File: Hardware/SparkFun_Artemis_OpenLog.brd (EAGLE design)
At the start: 30.5 x 30.5 mm, 126 parts, among them J14 CORTEX_JTAG, J6 MICRO-SD, Q1 20V/0.2A/8MHz/1.2Ω/1Vth, Q10 20V/0.2A/8MHz/1.2Ω/1Vth, Q2 20V/4.2A/52mΩ/1.4W, Q3 20V/0.2A/8MHz/1.2Ω/1Vth, Q7 20V/0.2A/8MHz/1.2Ω/1Vth, Q9 20V/0.2A/8MHz/1.2Ω/1Vth, U1 3.0V Supervisor, U10 CH340E, U13 ICM-20948, U14 1.8V/100mA, U2 MCP73831, U3 AP2112K, U4 AP2112K, U8 ARTEMIS_MODULE, Y3 32.768kHz

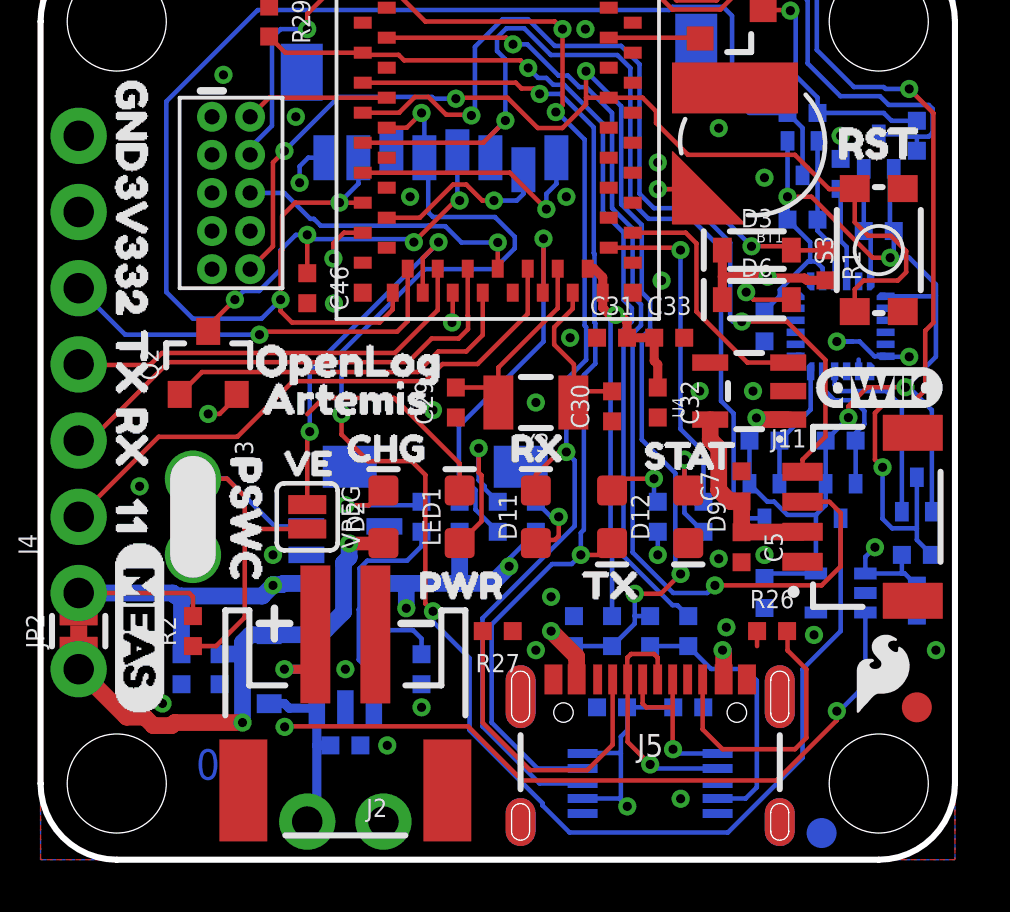
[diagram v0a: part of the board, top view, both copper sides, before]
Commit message: Update SparkFun_Artemis_OpenLog.brd
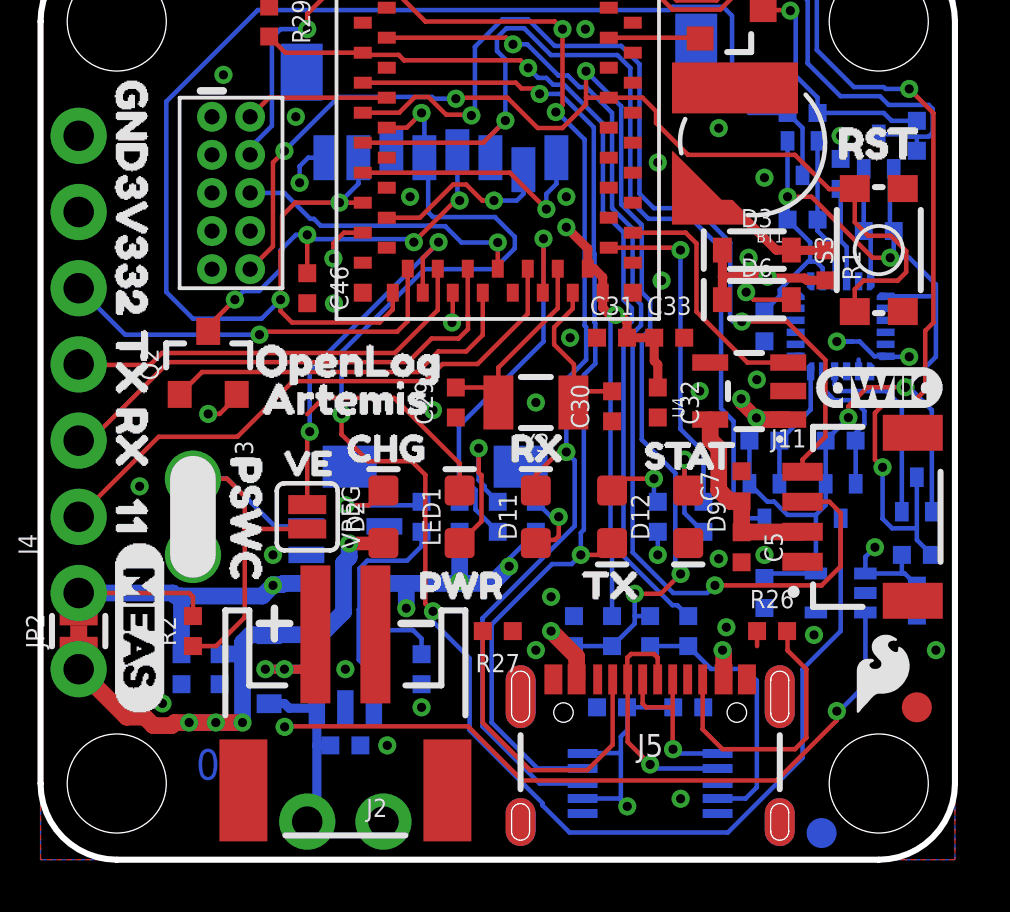
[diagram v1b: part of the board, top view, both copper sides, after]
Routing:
- net VCC_1: track 26.9 -> 33.2 mm, vias 2 -> 4
- net N$1: track 7.88 -> 5.07 mm, vias 2 -> 0
- net 5V: track 20.7 -> 22.5 mm, vias 4 -> 6
- net V_BATT: track 10.3 -> 11.6 mm, vias 1 -> 2
- net VIN: track 16.1 -> 17.0 mm, vias 2 -> 3
- net 3.3V: vias 8 -> 9
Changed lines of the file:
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@@
 <layers>
 <layer number="1" name="Top" color="4" fill="1" visible="yes" active="yes"/>
-<layer number="2" name="Vertical" color="1" fill="3" visible="no" active="yes"/>
-<layer number="15" name="Horz" color="4" fill="6" visible="no" active="yes"/>
+<layer number="2" name="Vertical" color="1" fill="3" visible="yes" active="yes"/>
+<layer number="15" name="Horz" color="4" fill="6" visible="yes" active="yes"/>
 <layer number="16" name="Bottom" color="1" fill="1" visible="yes" active="yes"/>
 <layer number="17" name="Pads" color="2" fill="1" visible="yes" active="yes"/>
@@
 <layer number="19" name="Unrouted" color="6" fill="1" visible="yes" active="yes"/>
 <layer number="20" name="Dimension" color="24" fill="1" visible="yes" active="yes"/>
-<layer number="21" name="tPlace" color="16" fill="1" visible="yes" active="yes"/>
-<layer number="22" name="bPlace" color="14" fill="1" visible="yes" active="yes"/>
-<layer number="23" name="tOrigins" color="15" fill="1" visible="yes" active="yes"/>
-<layer number="24" name="bOrigins" color="15" fill="1" visible="yes" active="yes"/>
+<layer number="21" name="tPlace" color="16" fill="1" visible="no" active="yes"/>
+<layer number="22" name="bPlace" color="14" fill="1" visible="no" active="yes"/>
+<layer number="23" name="tOrigins" color="15" fill="1" visible="no" active="yes"/>
+<layer number="24" name="bOrigins" color="15" fill="1" visible="no" active="yes"/>
 <layer number="25" name="tNames" color="7" fill="1" visible="no" active="yes"/>
 <layer number="26" name="bNames" color="7" fill="1" visible="no" active="yes"/>
@@
 <layer number="43" name="vRestrict" color="2" fill="10" visible="no" active="yes"/>
 <layer number="44" name="Drills" color="7" fill="1" visible="no" active="yes"/>
-<layer number="45" name="Holes" color="7" fill="1" visible="yes" active="yes"/>
+<layer number="45" name="Holes" color="7" fill="1" visible="no" active="yes"/>
 <layer number="46" name="Milling" color="3" fill="1" visible="no" active="yes"/>
 <layer number="47" name="Measures" color="7" fill="1" visible="no" active="yes"/>
 <layer number="48" name="Document" color="7" fill="1" visible="no" active="yes"/>
-<layer number="49" name="Reference" color="7" fill="1" visible="yes" active="yes"/>
+<layer number="49" name="Reference" color="7" fill="1" visible="no" active="yes"/>
 <layer number="50" name="dxf" color="7" fill="1" visible="no" active="yes"/>
-<layer number="51" name="tDocu" color="6" fill="1" visible="yes" active="yes"/>
+<layer number="51" name="tDocu" color="6" fill="1" visible="no" active="yes"/>
 <layer number="52" name="bDocu" color="7" fill="1" visible="no" active="yes"/>
 <layer number="91" name="Nets" color="2" fill="1" visible="no" active="no"/>
@@
 <contactref element="C7" pad="2"/>
 <contactref element="U4" pad="2"/>
-<via x="23.749" y="15.621" extent="1-16" drill="0.3048"/>
+<via x="23.876" y="16.002" extent="1-16" drill="0.3048"/>
 <contactref element="R3" pad="1"/>
 <wire x1="11.43" y1="1.27" x2="-4.31" y2="-29.21" width="0" layer="19" extent="1-1"/>
@@
 <wire x1="23.76838125" y1="18.669" x2="23.5204" y2="18.91698125" width="0.1524" layer="1"/>
 <via x="23.5204" y="18.91698125" extent="1-16" drill="0.3048"/>
+<via x="13.97" y="9.271" extent="1-16" drill="0.3048"/>
 </signal>
 <signal name="VIN" class="1">
@@
 <vertex x="0" y="10.16"/>
 </polygon>
+<via x="23.35554375" y="15.3622" extent="1-16" drill="0.3048"/>
+<wire x1="23.35554375" y1="15.3622" x2="23.35554375" y2="15.2352" width="0.4572" layer="1"/>
+<wire x1="23.35554375" y1="15.2352" x2="23.86354375" y2="14.7272" width="0.4572" layer="1"/>
 </signal>
 <signal name="N$7">
@@
 <wire x1="9.017" y1="6.35" x2="9.16" y2="6.493" width="0.1524" layer="1"/>
 <wire x1="8.89" y1="6.35" x2="8.128" y2="6.35" width="0.3048" layer="16"/>
+<via x="7.493" y="6.35" extent="1-16" drill="0.3048"/>
+<wire x1="7.493" y1="6.35" x2="8.128" y2="6.35" width="0.3048" layer="1"/>
+<wire x1="7.493" y1="6.35" x2="8.128" y2="6.35" width="0.3048" layer="16"/>
 </signal>
 <signal name="ARTEMIS_SWDIO">
@@
 <wire x1="22.77" y1="6.01" x2="22.77" y2="6.948" width="0.5588" layer="1"/>
 <wire x1="22.77" y1="6.948" x2="22.733" y2="6.985" width="0.5588" layer="1"/>
+<via x="5.842" y="4.572" extent="1-16" drill="0.3048"/>
+<wire x1="5.842" y1="4.572" x2="6.731" y2="4.572" width="0.5588" layer="16"/>
+<via x="4.953" y="4.572" extent="1-16" drill="0.3048"/>
+<wire x1="4.953" y1="4.572" x2="5.842" y2="4.572" width="0.5588" layer="16"/>
 </signal>
 <signal name="N$25">
@@
 <wire x1="22.6822" y1="20.3765625" x2="21.6973625" y2="21.3614" width="0.1524" layer="16"/>
 <contactref element="J6" pad="DI"/>
-<wire x1="23.1014" y1="11.8236" x2="23.1014" y2="14.8716" width="0.1524" layer="16"/>
-<wire x1="23.1014" y1="14.8716" x2="22.6822" y2="15.2908" width="0.1524" layer="16"/>
-<wire x1="22.6822" y1="15.2908" x2="22.6822" y2="20.3765625" width="0.1524" layer="16"/>
+<wire x1="23.1014" y1="11.8236" x2="23.1014" y2="14.6176" width="0.1524" layer="16"/>
+<wire x1="23.1014" y1="14.6176" x2="22.6822" y2="15.0368" width="0.1524" layer="16"/>
+<wire x1="22.6822" y1="15.0368" x2="22.6822" y2="20.3765625" width="0.1524" layer="16"/>
 <wire x1="15.494" y1="26.67905625" x2="15.2146" y2="26.95845625" width="0.1524" layer="16"/>
 <wire x1="15.2146" y1="26.95845625" x2="15.2146" y2="27.40034375" width="0.1524" layer="16"/>
@@
 <contactref element="R1" pad="1"/>
 <contactref element="D3" pad="A"/>
-<wire x1="25.026" y1="20.32" x2="25.273" y2="20.32" width="0.1524" layer="1"/>
-<wire x1="25.281" y1="20.312" x2="26.162" y2="20.312" width="0.1524" layer="1"/>
-<wire x1="25.273" y1="20.32" x2="25.281" y2="20.312" width="0.1524" layer="1"/>
-<wire x1="25.026" y1="20.32" x2="24.899" y2="20.447" width="0.1524" layer="1"/>
-<wire x1="24.899" y1="20.447" x2="23.6982" y2="20.447" width="0.1524" layer="1"/>
-<via x="23.6982" y="20.447" extent="1-16" drill="0.3048"/>
-<wire x1="21.727" y1="21.981" x2="21.727" y2="21.844" width="0.1524" layer="1"/>
-<wire x1="21.7932" y1="22.352" x2="20.574" y2="22.352" width="0.1524" layer="16"/>
-<via x="20.574" y="22.352" extent="1-16" drill="0.3048"/>
-<wire x1="20.574" y1="22.352" x2="21.356" y2="22.352" width="0.1524" layer="1"/>
-<wire x1="21.356" y1="22.352" x2="21.727" y2="21.981" width="0.1524" layer="1"/>
-<wire x1="23.6982" y1="20.447" x2="21.7932" y2="22.352" width="0.1524" layer="16"/>
+<wire x1="21.727" y1="21.844" x2="22.99805" y2="21.844" width="0.3048" layer="1"/>
+<wire x1="24.52205" y1="20.32" x2="25.026" y2="20.32" width="0.3048" layer="1"/>
+<wire x1="22.99805" y1="21.844" x2="24.52205" y2="20.32" width="0.3048" layer="1"/>
+<wire x1="26.162" y1="20.312" x2="25.034" y2="20.312" width="0.3048" layer="1"/>
+<wire x1="25.034" y1="20.312" x2="25.026" y2="20.32" width="0.3048" layer="1"/>
 </signal>
 <signal name="VCC_1">
@@
 <wire x1="24.235" y1="19.431" x2="23.8684875" y2="19.431" width="0.3048" layer="1"/>
 <wire x1="23.8684875" y1="19.431" x2="23.77290625" y2="19.52658125" width="0.3048" layer="1"/>
-<wire x1="23.77290625" y1="19.52658125" x2="23.26789375" y2="19.52658125" width="0.3048" layer="1"/>
+<wire x1="23.77290625" y1="19.52658125" x2="23.622" y2="19.52658125" width="0.3048" layer="1"/>
+<wire x1="23.622" y1="19.52658125" x2="23.26789375" y2="19.52658125" width="0.3048" layer="1"/>
 <wire x1="23.26789375" y1="19.52658125" x2="23.1723125" y2="19.431" width="0.3048" layer="1"/>
 <wire x1="23.1723125" y1="19.431" x2="22.726" y2="19.431" width="0.3048" layer="1"/>
@@
 <wire x1="18.99994375" y1="17.98394375" x2="19.177" y2="18.161" width="0.1524" layer="16"/>
 <wire x1="18.99994375" y1="10.36394375" x2="18.99994375" y2="17.98394375" width="0.1524" layer="16"/>
-<wire x1="24.0795125" y1="19.65358125" x2="23.2152875" y2="19.65358125" width="0.5588" layer="15"/>
+<wire x1="24.0795125" y1="19.65358125" x2="23.622" y2="19.65358125" width="0.5588" layer="15"/>
+<wire x1="23.622" y1="19.65358125" x2="23.2152875" y2="19.65358125" width="0.5588" layer="15"/>
 <wire x1="24.235" y1="19.431" x2="24.235" y2="19.49809375" width="0.5588" layer="15"/>
 <wire x1="24.235" y1="19.49809375" x2="24.0795125" y2="19.65358125" width="0.5588" layer="15"/>
 <wire x1="21.72270625" y1="18.161" x2="19.177" y2="18.161" width="0.5588" layer="15"/>
 <wire x1="23.2152875" y1="19.65358125" x2="21.72270625" y2="18.161" width="0.5588" layer="15"/>
+<via x="23.6" y="20.066" extent="1-16" drill="0.3048"/>
+<wire x1="23.6" y1="20.066" x2="23.6" y2="19.54858125" width="0.3048" layer="1"/>
+<wire x1="23.6" y1="19.54858125" x2="23.622" y2="19.52658125" width="0.3048" layer="1"/>
+<wire x1="23.6" y1="20.066" x2="23.6" y2="19.67558125" width="0.5588" layer="15"/>
+<wire x1="23.6" y1="19.67558125" x2="23.622" y2="19.65358125" width="0.3048" layer="15"/>
+<via x="17.526" y="21.082" extent="1-16" drill="0.3048"/>
+<wire x1="17.526" y1="21.082" x2="17.526" y2="19.812" width="0.5588" layer="15"/>
+<wire x1="17.526" y1="19.812" x2="19.177" y2="18.161" width="0.5588" layer="15"/>
+<wire x1="17.526" y1="21.082" x2="18.24" y2="20.368" width="0.3048" layer="1"/>
+<wire x1="18.24" y1="20.368" x2="18.24" y2="19.7" width="0.3048" layer="1"/>
 </signal>
 <signal name="!POWER_LOSS!">
